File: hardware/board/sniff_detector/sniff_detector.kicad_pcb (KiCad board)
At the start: 2 copper layers, 51 x 21 mm, 27 parts, among them J1 Conn_01x20_Female, J2 Conn_01x20_Female, J3 Conn_Coaxial, J4 Conn_01x03_Female, U1 AD8226, U2 REF2033

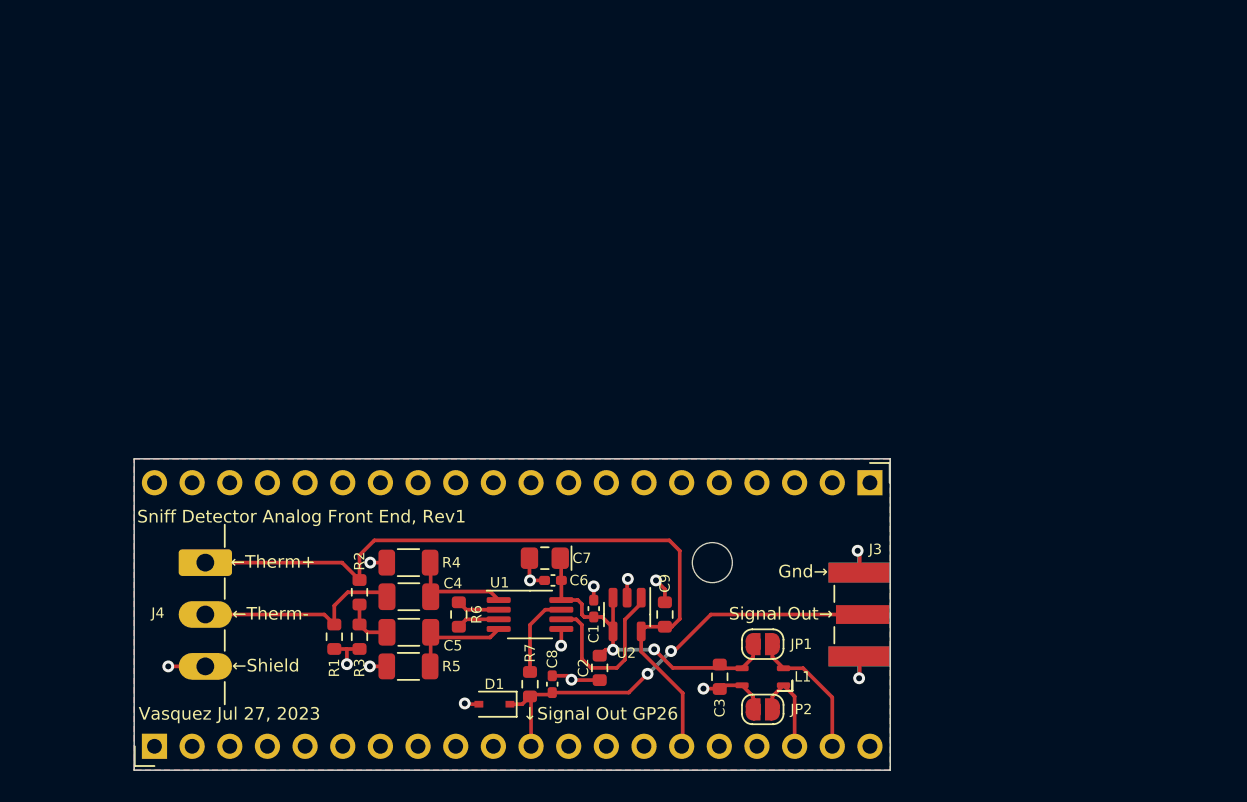
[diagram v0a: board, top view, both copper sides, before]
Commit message: complete pcb v0.2
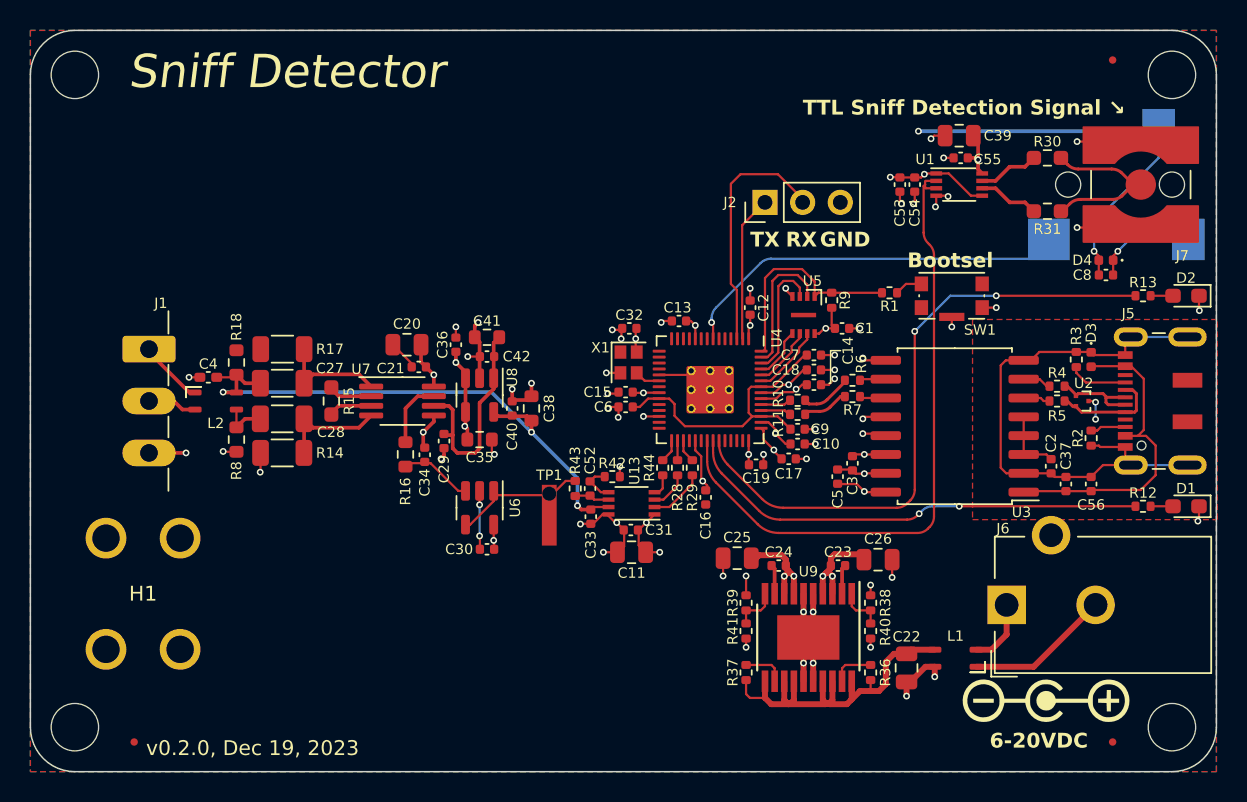
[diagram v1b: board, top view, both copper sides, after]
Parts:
- removed the J1 at (172.1, 84.0)
- removed J3: Conn_Coaxial, Connector_Coaxial:SMA_Samtec_SMA-J-P-X-ST-EM1_EdgeMount
- removed JP1, JP2: Jumper_2_Open, Jumper:SolderJumper-2_P1.3mm_Open_RoundedPad1.0x1.5mm
- added C1: 100nF, Capacitor_SMD:C_0402_1005Metric, F.Cu at (170.2, 73.6)
- added C10: 1uF, Capacitor_SMD:C_0402_1005Metric, F.Cu at (167.2, 81.4)
- added C11: 10uF, Capacitor_SMD:C_0805_2012Metric, F.Cu at (156.1, 88.7)
- added C12: 100nF, Capacitor_SMD:C_0402_1005Metric, F.Cu at (164.1, 72.2)
- added C13: 100nF, Capacitor_SMD:C_0402_1005Metric, F.Cu at (159.2, 73.1)
- added C14: 100nF, Capacitor_SMD:C_0402_1005Metric, F.Cu at (168.3, 77.4)
- added C15: 100nF, Capacitor_SMD:C_0402_1005Metric, F.Cu at (155.7, 77.9)
- added C16: 100nF, Capacitor_SMD:C_0402_1005Metric, F.Cu at (161.1, 85.0)
- added C17: 100nF, Capacitor_SMD:C_0402_1005Metric, F.Cu at (166.7, 82.4)
- added C18: 100nF, Capacitor_SMD:C_0402_1005Metric, F.Cu at (168.3, 76.4)
- added C19: 100nF, Capacitor_SMD:C_0402_1005Metric, F.Cu at (164.4, 82.8)
- added C22: 3.3uF, Capacitor_SMD:C_0805_2012Metric, F.Cu at (174.6, 96.5)
- added C23: 10nF, Capacitor_SMD:C_0402_1005Metric, F.Cu at (170.0, 89.6)
- added C24: 10nF, Capacitor_SMD:C_0402_1005Metric, F.Cu at (166.0, 89.6)
- added C25: 10uF, Capacitor_SMD:C_0805_2012Metric, F.Cu at (163.2, 89.1)
- added C26: 22uF, Capacitor_SMD:C_0805_2012Metric, F.Cu at (172.7, 89.2)
- added C29: 100nF, Capacitor_SMD:C_0402_1005Metric, F.Cu at (143.4, 81.2)
- added C30: 100nF, Capacitor_SMD:C_0402_1005Metric, F.Cu at (146.3, 88.5)
- added C31: 100nF, Capacitor_SMD:C_0402_1005Metric, F.Cu at (156.0, 87.2)
- added C32: 10nF, Capacitor_SMD:C_0402_1005Metric, F.Cu at (155.9, 73.6)
- added C33: 100nF, Capacitor_SMD:C_0402_1005Metric, F.Cu at (153.3, 86.3)
- added C35: 10uF, Resistor_SMD:R_0603_1608Metric, F.Cu at (145.8, 81.1)
- added C37: 100nF, Capacitor_SMD:C_0402_1005Metric, F.Cu at (185.3, 84.1)
- added C39: 10uF, Capacitor_SMD:C_0805_2012Metric, F.Cu at (178.2, 60.6)
- added C4: 1uF, Capacitor_SMD:C_0402_1005Metric_Pad0.74x0.62mm_HandSolder, F.Cu at (127.5, 76.9)
- added C40: 100nF, Capacitor_SMD:C_0402_1005Metric, F.Cu at (148.0, 79.0)
- added C41: 10uF, Resistor_SMD:R_0603_1608Metric, F.Cu at (146.3, 74.2)
- added C42: 100nF, Capacitor_SMD:C_0402_1005Metric, F.Cu at (146.3, 75.5)
- added C5: 100nF, Capacitor_SMD:C_0402_1005Metric, F.Cu at (169.9, 83.6)
- added C52: 300pF, Capacitor_SMD:C_0402_1005Metric, F.Cu at (153.2, 84.4)
- added C53: 1uF, Capacitor_SMD:C_0402_1005Metric, F.Cu at (174.2, 63.9)
- added C54: 100nF, Capacitor_SMD:C_0402_1005Metric, F.Cu at (175.2, 63.9)
- added C55: 100nF, Capacitor_SMD:C_0402_1005Metric, F.Cu at (178.2, 62.1)
- added C56: 1uF, Capacitor_SMD:C_0402_1005Metric, F.Cu at (187.1, 84.1)
- added C6: 100nF, Capacitor_SMD:C_0402_1005Metric, F.Cu at (155.7, 78.9)
- added C7: 100nF, Capacitor_SMD:C_0402_1005Metric, F.Cu at (168.3, 75.4)
- added C8: 1uF, Capacitor_SMD:C_0402_1005Metric, F.Cu at (188.1, 70.0)
- added C9: 1uF, Capacitor_SMD:C_0402_1005Metric, F.Cu at (167.2, 80.4)
- added D2: LED, LED_SMD:LED_0603_1608Metric_Pad1.05x0.95mm_HandSolder, F.Cu at (193.4, 71.4)
- added D3: D_TVS, Diode_SMD:D_0402_1005Metric, F.Cu at (187.1, 75.7)
- added D4: D_TVS, Diode_SMD:D_0402_1005Metric, F.Cu at (188.1, 69.0)
- added FID1: Fiducial, Fiducial:Fiducial_0.5mm_Mask1mm, F.Cu at (122.5, 101.5)
- added FID2: Fiducial, Fiducial:Fiducial_0.5mm_Mask1mm, F.Cu at (188.5, 101.5)
- added FID3: Fiducial, Fiducial:Fiducial_0.5mm_Mask1mm, F.Cu at (188.5, 55.5)
- added G***: LOGO, LOGO, B.Cu at (133.5, 65.4)
- added G3: LOGO, LOGO, F.Cu at (184.0, 98.7)
- added J4: AudioJack3, Connector_Audio:Jack_3.5mm_CUI_SJ-3523-SMT_Horizontal, B.Cu at (190.0, 63.9)
- added J5: USB_C_Receptacle_USB2.0, Connector_USB:USB_C_Receptacle_JAE_DX07S016JA1R1500, F.Cu at (192.4, 78.5)
- added J6: Barrel_Jack_Switch, Connector_BarrelJack:BarrelJack_CUI_PJ-102AH_Horizontal, F.Cu at (181.3, 92.2)
- added J7: Conn_Coaxial, kicad_component_library:SMA_TE_Connectivity_CONSMA002-SMD-G-T_Horizontal, F.Cu at (190.4, 63.9)
- added L2: L_Coupled_1423, kicad_component_library:L_CommonModeChoke_TDKCorporation_1210, F.Cu at (128.0, 78.5)
- added R1: 1K, Resistor_SMD:R_0402_1005Metric, F.Cu at (173.4, 71.2)
- added R10: 27, Resistor_SMD:R_0402_1005Metric, F.Cu at (167.2, 78.5)
- added R11: 27, Resistor_SMD:R_0402_1005Metric, F.Cu at (167.2, 79.4)
- added R12: 680, Resistor_SMD:R_0402_1005Metric, F.Cu at (190.6, 85.6)
- added R13: 680, Resistor_SMD:R_0402_1005Metric, F.Cu at (190.6, 71.4)
- added R17: 15M, Resistor_SMD:R_1206_3216Metric, F.Cu at (132.5, 75.0)
- added R18: 22K, Resistor_SMD:R_0603_1608Metric, F.Cu at (129.4, 75.9)
- added R28: 49.9, Resistor_SMD:R_0402_1005Metric, F.Cu at (159.2, 83.0)
- added R29: 49.9, Resistor_SMD:R_0402_1005Metric, F.Cu at (160.2, 83.0)
- added R30: 100, Resistor_SMD:R_0603_1608Metric_Pad0.98x0.95mm_HandSolder, F.Cu at (184.1, 62.1)
- added R31: 100, Resistor_SMD:R_0603_1608Metric_Pad0.98x0.95mm_HandSolder, F.Cu at (184.1, 65.7)
- added R36: 1M, Resistor_SMD:R_0402_1005Metric, F.Cu at (172.2, 96.8)
- added R37: 1M, Resistor_SMD:R_0402_1005Metric, F.Cu at (163.8, 96.8)
- added R38: 309K, Resistor_SMD:R_0402_1005Metric, F.Cu at (172.2, 92.1)
- added R39: 172K, Resistor_SMD:R_0402_1005Metric, F.Cu at (163.8, 92.1)
- added R40: 100K, Resistor_SMD:R_0402_1005Metric, F.Cu at (172.2, 94.0)
- added R41: 100K, Resistor_SMD:R_0402_1005Metric, F.Cu at (163.8, 94.0)
- added R42: 100, Resistor_SMD:R_0402_1005Metric, F.Cu at (154.8, 83.6)
- added R43: 100, Resistor_SMD:R_0402_1005Metric, F.Cu at (152.2, 84.4)
- added R44: 49.9, Resistor_SMD:R_0402_1005Metric, F.Cu at (158.2, 83.0)
- added R5: 24, Resistor_SMD:R_0402_1005Metric, F.Cu at (184.8, 78.5)
- added R6: 24, Resistor_SMD:R_0402_1005Metric, F.Cu at (170.9, 77.1)
- added R7: 24, Resistor_SMD:R_0402_1005Metric, F.Cu at (170.9, 78.2)
- added R9: 10K, Resistor_SMD:R_0402_1005Metric, F.Cu at (169.6, 71.7)
- added REF**: MountingHole_3.2mm_M3_DIN965, MountingHole:MountingHole_3.2mm_M3_DIN965, F.Cu at (192.5, 100.5)
- added REF**: MountingHole_3.2mm_M3_DIN965, MountingHole:MountingHole_3.2mm_M3_DIN965, F.Cu at (192.5, 56.5)
- added REF**: MountingHole_3.2mm_M3_DIN965, MountingHole:MountingHole_3.2mm_M3_DIN965, F.Cu at (118.5, 56.5)
- added REF**: MountingHole_3.2mm_M3_DIN965, MountingHole:MountingHole_3.2mm_M3_DIN965, F.Cu at (118.5, 100.5)
- added REF1: OSHW-Logo2_7.3x6mm_SilkScreen, Symbol:OSHW-Logo2_7.3x6mm_SilkScreen, B.Cu at (124.3, 100.3)
- added SW1: ~, kicad_component_library:SW_Push_1P1T-SH_NO_Vertical_Wuerth_WS-TASV, F.Cu at (177.7, 71.4)
- added TP1: TestPoint, kicad_component_library:TestPoint_Keystone_5027_Miniature, F.Cu at (150.5, 86.2)
- added U1: 74LVCH2T45DC, Package_SO:VSSOP-8_2.3x2mm_P0.5mm, F.Cu at (178.2, 63.9)
- added U13: ADS7049, Package_SO:VSSOP-8_2.3x2mm_P0.5mm, F.Cu at (156.1, 85.4)
- added U2: TPD2EUSB30, Package_TO_SOT_SMD:Texas_DRT-3, F.Cu at (186.4, 78.5)
- added U3: ADUM4160, Package_SO:SOIC-16W_7.5x10.3mm_P1.27mm, F.Cu at (177.8, 80.2)
- added U4: RP2040, kicad_component_library:RP2040-QFN-56, F.Cu at (161.3, 77.7)
- added U5: W25Q16JVUXIQ, kicad_component_library:Winbond-8USON-2x3mm, F.Cu at (167.7, 72.7)
- added U6: AD8615, Package_TO_SOT_SMD:TSOT-23-5, F.Cu at (145.8, 85.7)
- added U9: LT3030, Package_SO:ETSSOP-20-1EP_4.4x6.5mm_P0.65mm_EP3x4.2mm, F.Cu at (168.0, 94.5)
- added X1: ECS-TXO-2016, Crystal:Crystal_SMD_2016-4Pin_2.0x1.6mm, F.Cu at (155.8, 75.9)
- C2, C3: value 10uF -> 100nF; footprint Resistor_SMD:R_0603_1608Metric -> Capacitor_SMD:C_0402_1005Metric
- C20: renamed from C7; footprint Capacitor_SMD:C_0805_2012Metric_Pad1.18x1.45mm_HandSolder -> Capacitor_SMD:C_0805_2012Metric
- C21: renamed from C6; value 0.1uF -> 100nF; footprint Capacitor_SMD:C_0402_1005Metric_Pad0.74x0.62mm_HandSolder -> Capacitor_SMD:C_0402_1005Metric
- C27: renamed from C4; value 0.1uF -> 0.01uF
- C28: renamed from C5; value 0.1uF -> 0.01uF
- C34: renamed from C8; value 1uF -> 100nF; footprint Capacitor_SMD:C_0402_1005Metric_Pad0.74x0.62mm_HandSolder -> Capacitor_SMD:C_0402_1005Metric
- C36: renamed from C1; value 0.1uF -> 100nF; footprint Capacitor_SMD:C_0402_1005Metric_Pad0.74x0.62mm_HandSolder -> Capacitor_SMD:C_0402_1005Metric
- D1: value D_Zener -> LED; footprint Diode_SMD:D_SOD-323 -> LED_SMD:LED_0603_1608Metric_Pad1.05x0.95mm_HandSolder
- H1: value MountingHole -> MountingHole_Pad; footprint MountingHole:MountingHole_2.7mm -> kicad_component_library:Terminal_Keystone_779x_EdgeMount_Horizontal
- J2: value Conn_01x20_Female -> Conn_01x03_Male; footprint Connector_PinHeader_2.54mm:PinHeader_1x20_P2.54mm_Vertical -> Connector_PinHeader_2.54mm:PinHeader_1x03_P2.54mm_Vertical
- L1: footprint machine_agency_components:L_CommonModeChoke_TDKCorporation_1210 -> kicad_component_library:L_CommonModeChoke_TDKCorporation_1210
- R15: renamed from R6; value 470 -> 499; footprint Resistor_SMD:R_0603_1608Metric -> Resistor_SMD:R_0603_1608Metric_Pad0.98x0.95mm_HandSolder
- R2, R3: value 22K -> 5K1; footprint Resistor_SMD:R_0603_1608Metric -> Resistor_SMD:R_0402_1005Metric
- R4: value 15M -> 24; footprint Resistor_SMD:R_1206_3216Metric -> Resistor_SMD:R_0402_1005Metric
- moved J2 55.2 mm to (165.1, 65.1)
- moved R3 51.8 mm to (186.1, 75.7), turned to 90 degrees
- moved R2 50.4 mm to (187.1, 81.0)
- moved D1 48.5 mm to (193.4, 85.6)
- moved R4 45.3 mm to (184.8, 77.5)
- moved H1 38.5 mm to (123.1, 91.5), turned to -90 degrees
- moved C2 33.3 mm to (184.3, 82.9), turned to 90 degrees
- moved C36 20.1 mm to (144.2, 74.7)
- moved U8 17.8 mm to (145.8, 78.1)
- moved C34 17.7 mm to (142.1, 82.1)
- moved R16 17.6 mm to (140.8, 82.1)
- moved C20 17.1 mm to (140.9, 74.7)
- moved C21 17.0 mm to (141.7, 76.2), turned to 0 degrees
- moved C3 17.0 mm to (170.9, 82.7), turned to 90 degrees
- moved R15 16.8 mm to (135.8, 78.5)
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- renumbered C9 to C38, J4 to J1, R5 to R14, R7 to R16, R1 to R8, U1 to U7, U2 to U8
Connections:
- net /+1V65 renamed VREF_1V65
- C2 pad 1: +5V -> GND1
- C2 pad 2: GNDA -> /Harp Core RP2040 + Isolated USB/VDD1
- C20 pad 2: GNDA -> GND
- C21 pad 1: +5V -> GND
- C21 pad 2: GNDA -> +5V
- C27 pad 1: Net-(C4-Pad1) -> VREF_3V3
- C27 pad 2: Net-(C4-Pad2) -> Net-(U7-IN-)
- C28 pad 1: Net-(C5-Pad1) -> Net-(C28-Pad1)
- C3 pad 1: +5V -> GND
- C3 pad 2: GNDA -> +3V3
- C34 pad 1: /VSIG -> /Sensing Front End/VSIG
- C34 pad 2: GNDA -> GND
- C36 pad 1: GNDA -> GND
- C38 pad 1: AVREF -> VREF_3V3
- C38 pad 2: GNDA -> GND
- D1 pad 1: /VSIG -> GND
- D1 pad 2: GNDA -> Net-(D1-A)
- J1 pad 1: AVREF -> Net-(J1-Pin_1)
- J1 pad 2: Net-(C4-Pad1) -> Net-(J1-Pin_2)
- J1 pad 3: GNDA -> GND
- J2 pad 1: unconnected-(J2-Pad1) -> /Harp Core RP2040 + Isolated USB/UART0_TXD
- J2 pad 2: unconnected-(J2-Pad2) -> /Harp Core RP2040 + Isolated USB/UART0_RXD
- J2 pad 3: unconnected-(J2-Pad3) -> GND
- L1 pad 1: GND -> GND2
- L1 pad 2: +5VP -> +12V
- L1 pad 3: +5V -> IN1
- L1 pad 4: GNDA -> GND
- R14 pad 2: GNDA -> GND
- R16 pad 2: /VSIG -> /Sensing Front End/VSIG
- R2 pad 1: AVREF -> Net-(J5-CC1)
- R2 pad 2: Net-(C5-Pad1) -> GND1
- R3 pad 1: Net-(C5-Pad1) -> Net-(J5-CC2)
- R3 pad 2: GNDA -> GND1
- R4 pad 1: Net-(C4-Pad2) -> /Harp Core RP2040 + Isolated USB/D+
- R4 pad 2: GNDA -> Net-(U3-UD+)
- R8 pad 1: Net-(C4-Pad1) -> Net-(C28-Pad1)
- R8 pad 2: GNDA -> GND
- U7 pad 1: Net-(C4-Pad2) -> Net-(U7-IN-)
- U7 pad 5: GNDA -> GND
- U8 pad 2: GNDA -> GND
- U8 pad 5: AVREF -> VREF_3V3
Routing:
- net GND: track 6.36 -> 97.8 mm, vias 0 -> 60
- net +3V3: track 0.00 -> 86.2 mm, vias 0 -> 26
- net AVREF: track 51.4 -> 0.00 mm
- net /Harp Core RP2040 + Isolated USB/TTL_OUT: track 0.00 -> 44.2 mm
- net Net-(U4-GPIO25): track 0.00 -> 42.7 mm, vias 0 -> 2
- net GND1: track 0.00 -> 39.8 mm, vias 0 -> 2
- net VREF_3V3: track 0.00 -> 39.4 mm, vias 0 -> 3
- net Net-(U4-GPIO24): track 0.00 -> 31.7 mm, vias 0 -> 2
- net GNDA: track 30.0 -> 0.00 mm, vias 14 -> 0
- net /VSIG: track 29.7 -> 0.00 mm, vias 2 -> 0
- net /Harp Core RP2040 + Isolated USB/HARP_CLK_SYNC: track 0.00 -> 26.5 mm, vias 0 -> 1
- net IN1: track 0.00 -> 26.1 mm
- net VBUS: track 0.00 -> 21.6 mm
- net +1V1: track 0.00 -> 19.6 mm
- net /Harp Core RP2040 + Isolated USB/UART0_RXD: track 0.00 -> 16.6 mm
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- added copper zone on In2.Cu, net +3V3
- added copper zone on In2.Cu, net +5V
- added copper zone on B.Cu, net GND
- added copper zone on F.Cu, net GND
- added copper zone on In1.Cu, net GND
- added copper zone on F.Cu, net GND1
- removed copper zone on B.Cu, net GNDA
- removed copper zone on F.Cu, net GNDA
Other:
- board size 51 x 21 mm -> 80 x 50 mm
- copper layers 2 -> 4
- board text added: "6-20VDC"
- board text added: "Bootsel"
- board text added: "Chassis Ground"
- board text added: "Fits in enclosure: 1455C801"
- board text added: "Harp Sync Input ↑"
- board text added: "Isolated USB"
- board text added: "RX"
- board text added: "Shield (Gnd)"
- board text added: "Sniff Detector"
- board text added: "Sniff detection implant companion board"
- board text added: "Sonya Vasquez"
- board text added: "Source Files & Setup ↓"
- board text added: "TTL Sniff Detection Signal ↘"
- board text added: "TX"
- board text added: "Therm+"
- board text added: "Therm-"
- board text added: "v0.2.0, Dec 19, 2023"
- board text removed: "3v3"
- board text removed: "AGND"
- board text removed: "Gnd→"
- board text removed: "Signal Out→"
- board text removed: "Sniff Detector Analog Front End, Rev1"
- board text removed: "VSYS"
- board text removed: "Vasquez Jul 27, 2023"
- board text removed: "←Shield"
- board text removed: "←Therm+"
- board text removed: "←Therm-"
- board text removed: "↓Signal Out GP26"
